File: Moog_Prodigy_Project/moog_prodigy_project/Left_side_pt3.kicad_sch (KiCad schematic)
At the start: 68 parts, among them J1 P2-3, J2 P2-4, J3 P2-2, J4 P2-1, J5 P2-1, SW6 Switch_1x3, SW7 Switch_4x4, SW8 SW_Slide_DPDT_3x3, U10 NE5532, U11 OPA234, U12 OPA134, U13 NE5532, U14 OPA134, U9 NE5532

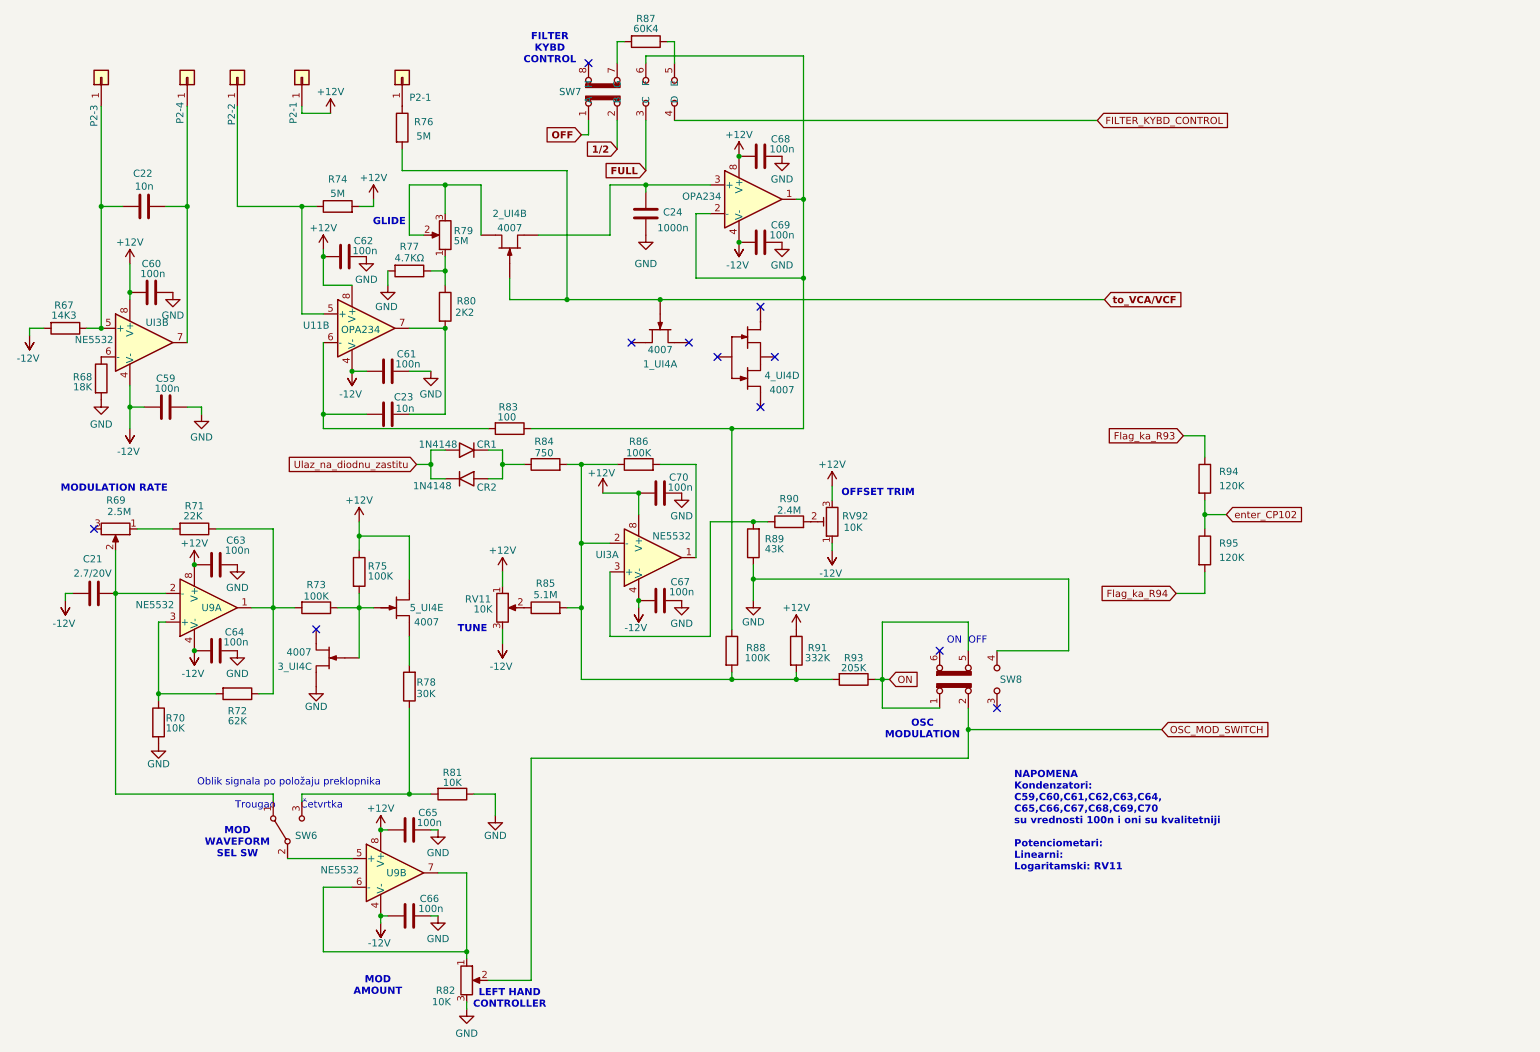
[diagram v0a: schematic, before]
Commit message: Update seme final 1
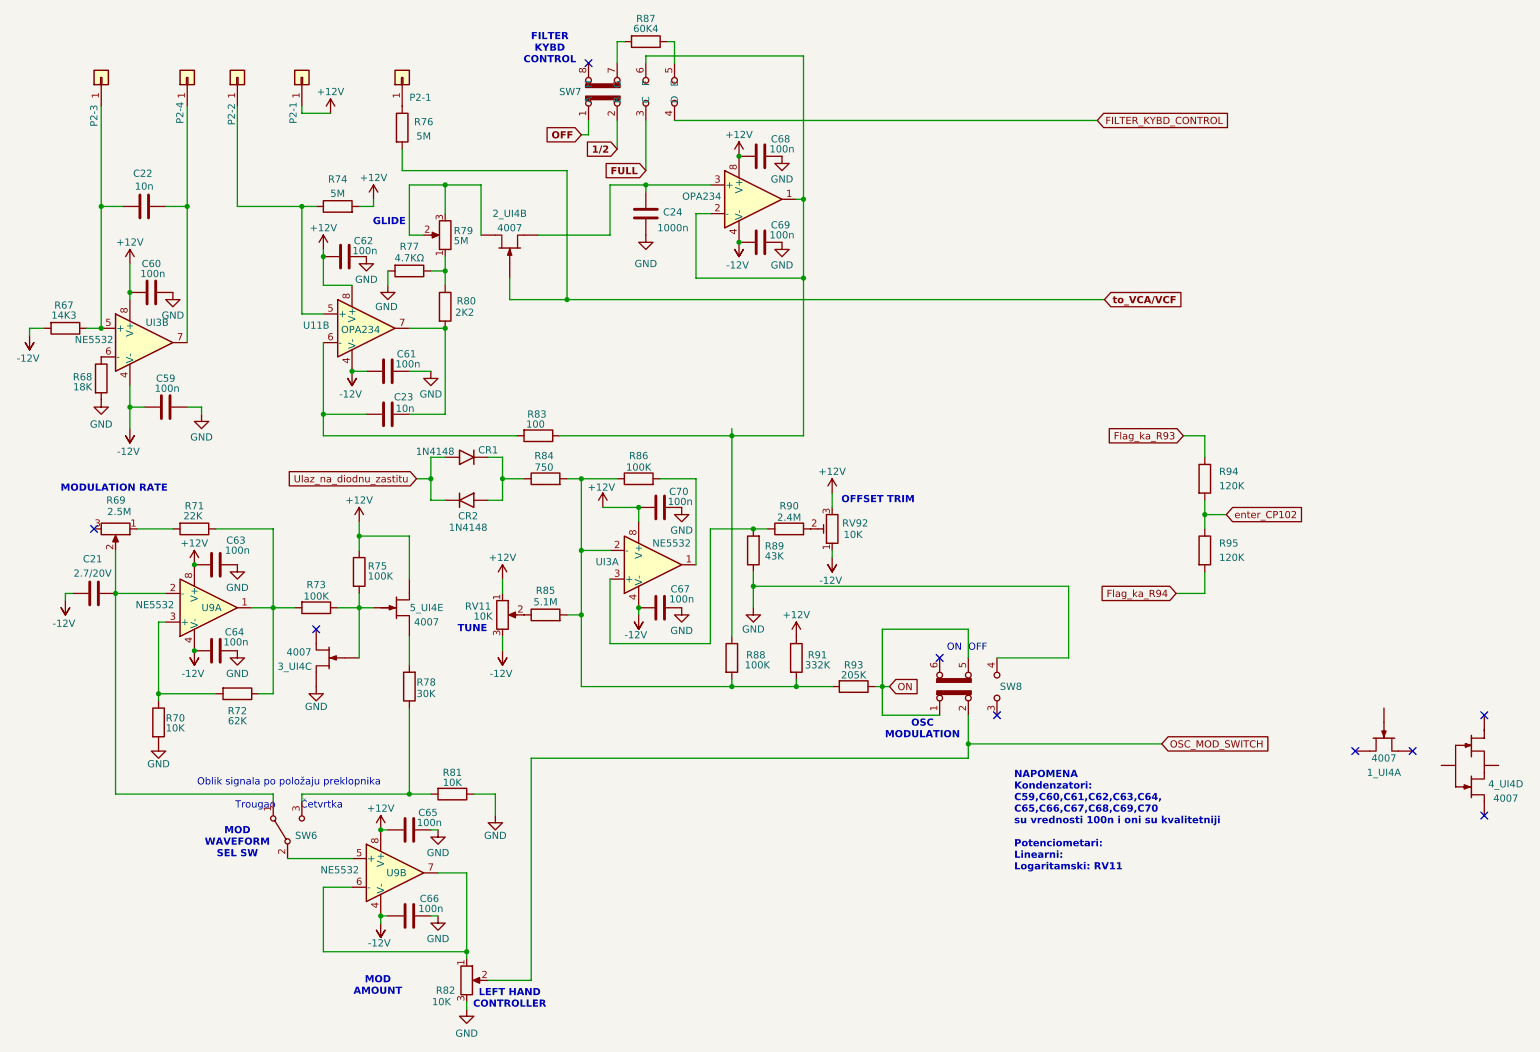
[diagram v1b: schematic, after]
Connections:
- net to_VCA/VCF: no longer 1_UI4.
- no-connect marks 11 -> 9
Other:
- moved on the sheet: 1_UI4A, 4_UI4D, C67, C70, CR1, CR2, R83, R84, R85, R86, R88, R89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
